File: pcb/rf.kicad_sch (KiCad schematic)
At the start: 51 parts, among them J4 Conn_Coaxial, J5 Conn_Coaxial, U5 NEO-M9N

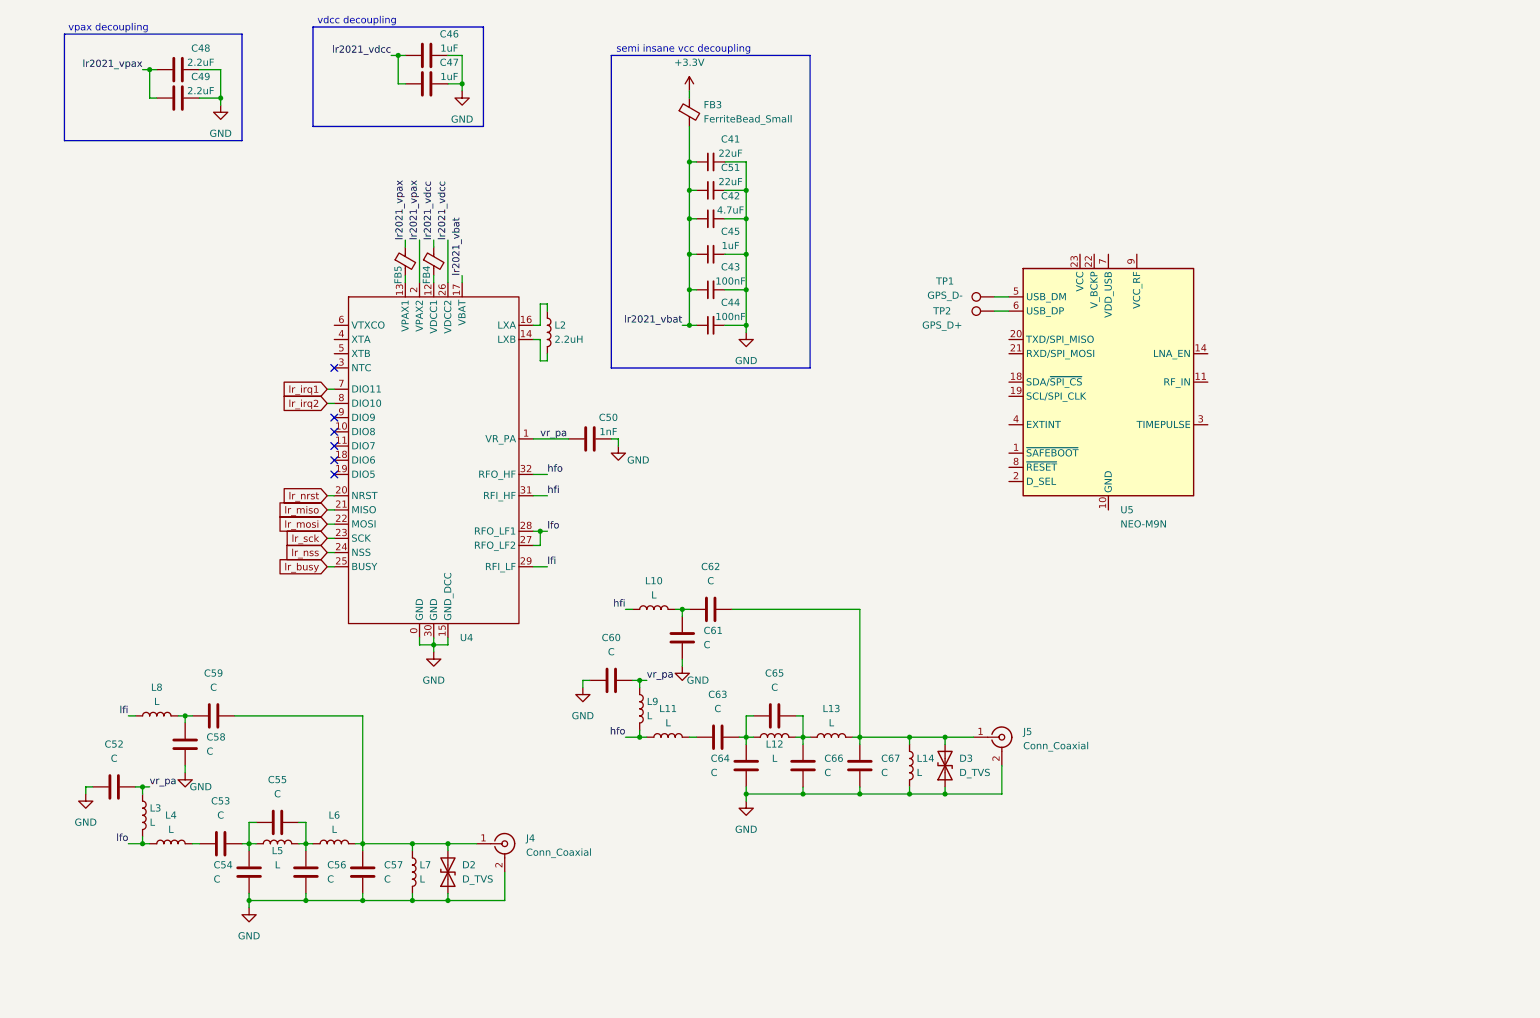
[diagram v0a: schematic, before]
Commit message: added missing files, rf stuff done I think (hope)
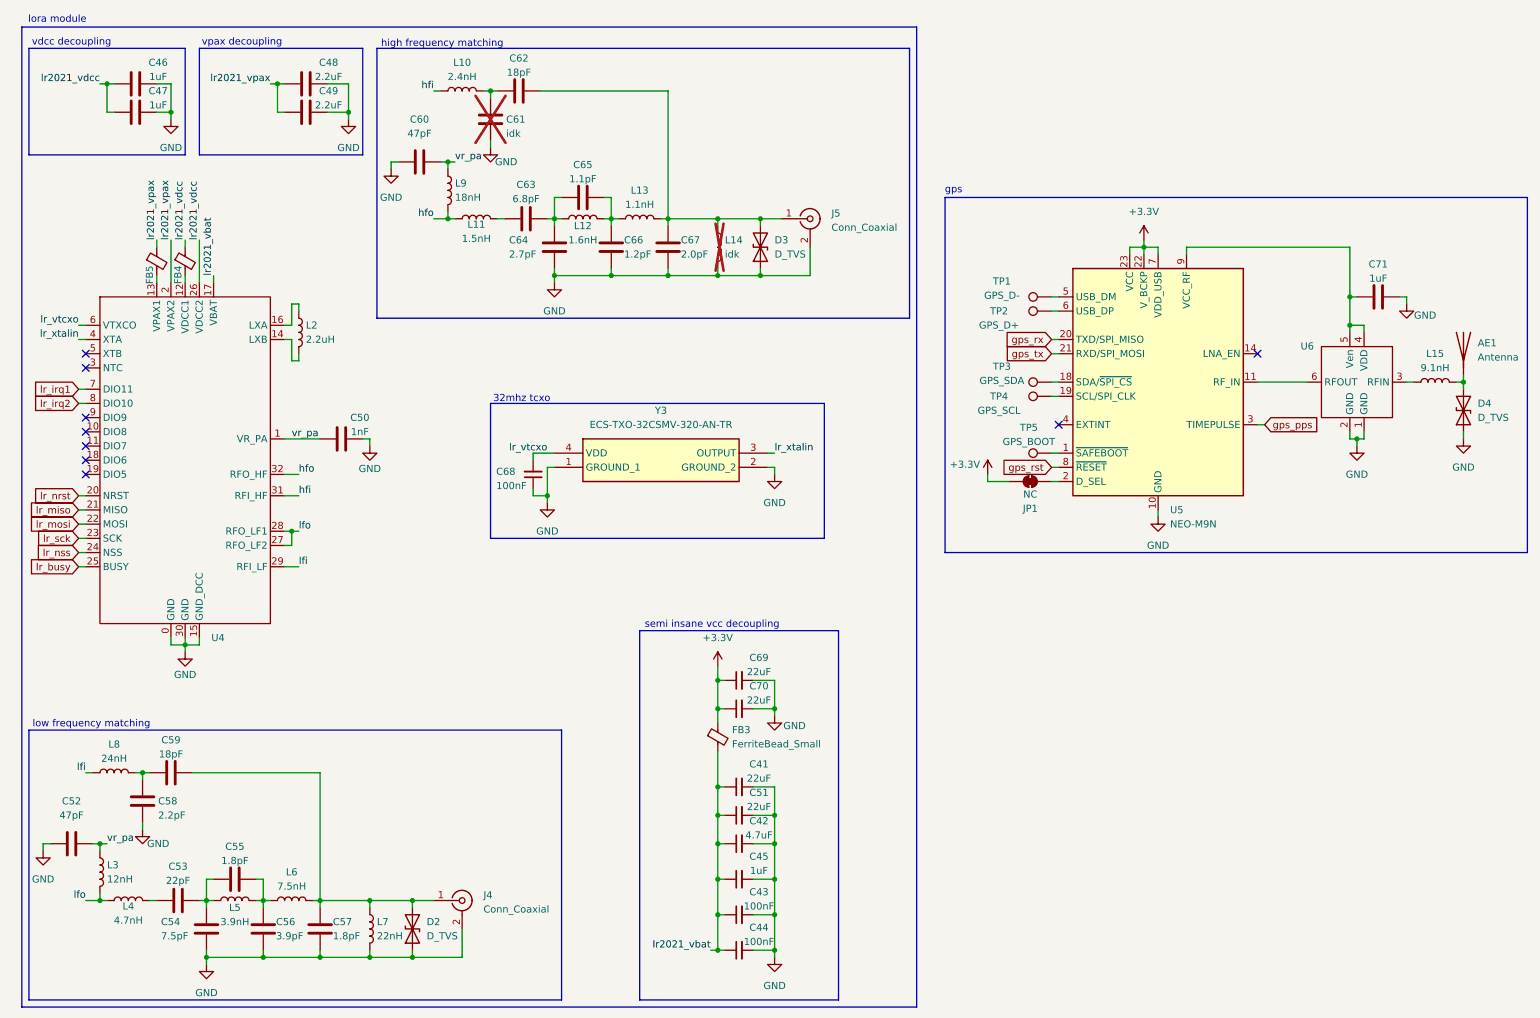
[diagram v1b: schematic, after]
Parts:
- added AE1: Antenna, symbol Device:Antenna
- added C68: 100nF, symbol Device:C_Small
- added C69, C70: 22uF, symbol Device:C_Small
- added C71: 1uF, symbol Device:C
- added D4: D_TVS, symbol Device:D_TVS
- added JP1: NC, symbol Jumper:SolderJumper_2_Bridged
- added L15: 9.1nH, symbol Device:L
- added TP3: GPS_SDA, symbol Connector:TestPoint
- added TP4: GPS_SCL, symbol Connector:TestPoint
- added TP5: GPS_BOOT, symbol Connector:TestPoint
- added U6: ~, symbol alnd-wb-0013-t:ALND-WB-0013-T
- added Y3: ECS-TXO-32CSMV-320-AN-TR, ECSTXO32CSMV320ANTR, symbol ECS-TXO-32CSMV-320-AN-TR:ECS-TXO-32CSMV-320-AN-TR
- C52, C60: value C -> 47pF
- C53: value C -> 22pF
- C54: value C -> 7.5pF
- C55, C57: value C -> 1.8pF
- C56: value C -> 3.9pF
- C58: value C -> 2.2pF
- C59, C62: value C -> 18pF
- C61: value C -> idk; now not fitted
- C63: value C -> 6.8pF
- C64: value C -> 2.7pF
- C65: value C -> 1.1pF
- C66: value C -> 1.2pF
- C67: value C -> 2.0pF
- L10: value L -> 2.4nH
- L11: value L -> 1.5nH
- L12: value L -> 1.6nH
- L13: value L -> 1.1nH
- L14: value L -> idk; now not fitted
- L3: value L -> 12nH
- L4: value L -> 4.7nH
- L5: value L -> 3.9nH
- L6: value L -> 7.5nH
- L7: value L -> 22nH
- L8: value L -> 24nH
- L9: value L -> 18nH
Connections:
- net +3.3V: now also U5.22 (V_BCKP), U5.23 (VCC), U5.7 (VDD_USB), C69.1, C70.1, JP1.1 (A)
- net GND: now also U5.10 (GND), U5.12 (GND), U5.13 (GND), U5.24 (GND), C68.1, C69.2, C70.2, C71.2, D4.1 (A1), U6.1 (GND), U6.2 (GND), Y3.1 (GROUND_1), Y3.2 (GROUND_2)
- net lr_xtalin: now reaches U4.4 (XTA)
- net lr_xtalin: now also Y3.3 (OUTPUT)
- net lr_vtcxo: now reaches U4.6 (VTXCO)
- net lr_vtcxo: now also C68.2, Y3.4 (VDD)
- net at U5.1 (~{SAFEBOOT}): now also TP5.1
- net at U5.11 (RF_IN): now also U6.6 (RFOUT)
- net at U5.18 (SDA/~{SPI_CS}): now also TP3.1
- net at U5.19 (SCL/SPI_CLK): now also TP4.1
- net at U5.2 (D_SEL): now also JP1.2 (B)
- net gps_rx: now reaches U5.20 (TXD/SPI_MISO)
- net gps_tx: now reaches U5.21 (RXD/SPI_MOSI)
- net gps_pps: now reaches U5.3 (TIMEPULSE)
- net gps_rst: now reaches U5.8 (~{RESET})
- net at U5.9 (VCC_RF): now also C71.1, U6.4 (VDD), U6.5 (Ven)
- new net: AE1.1 (A), D4.2 (A2), L15.2
- new net: L15.1, U6.3 (RFIN)
- no-connect marks 6 -> 9
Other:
- note added: "32mhz tcxo"
- note added: "gps"
- note added: "high frequency matching"
- note added: "lora module"
- note added: "low frequency matching"
- moved on the sheet: C41, C42, C43, C44, C45, C46, C47, C48, C49, C50, C51, C52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
